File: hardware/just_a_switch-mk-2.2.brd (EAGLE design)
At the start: 22.9 x 17.8 mm, 13 parts, among them U1_ ROTARY_ENCODER_SWITCH, U2 Tiny85

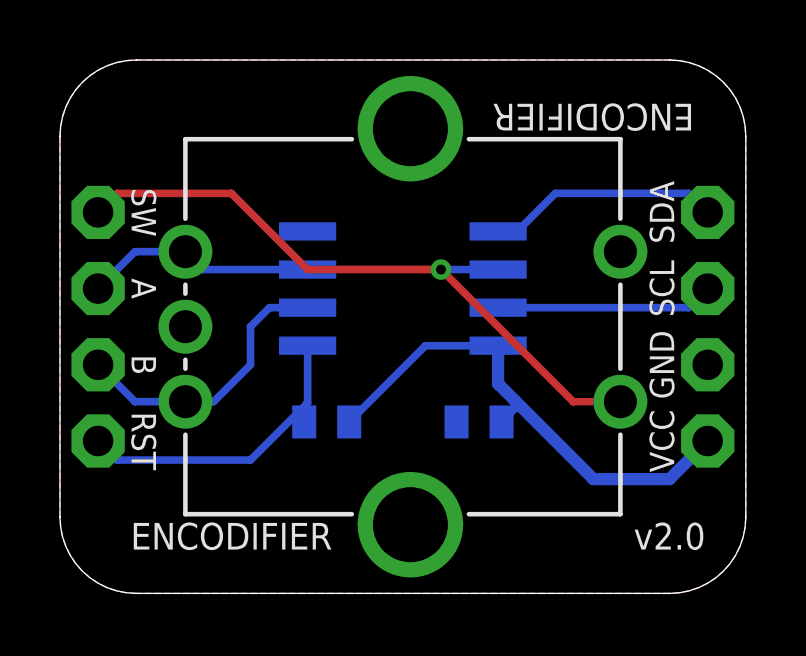
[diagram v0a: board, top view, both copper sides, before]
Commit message: have some boards, dawg
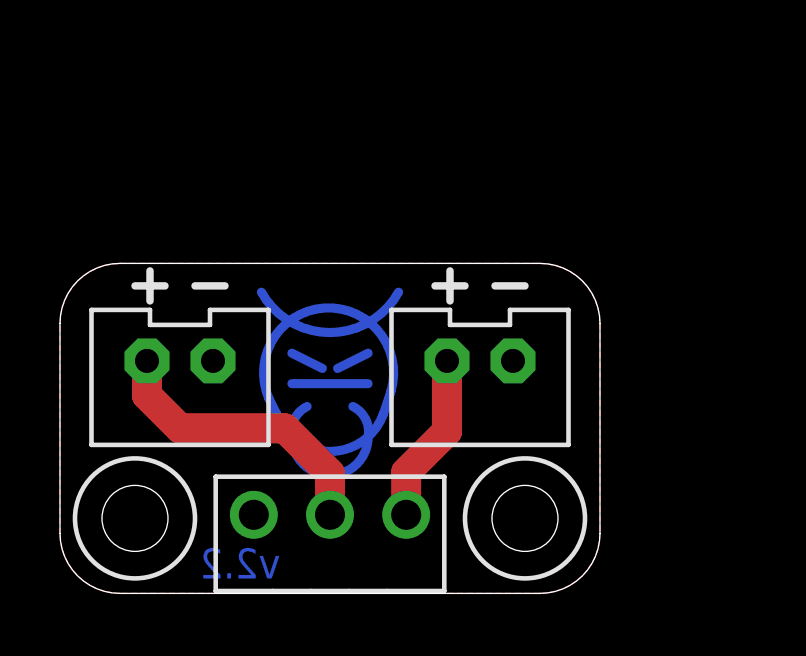
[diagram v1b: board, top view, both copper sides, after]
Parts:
- removed A, B, GND, RST, SCL, SDA, SW, VCC: M01PTH-1MM, a_parts:1X01-1MM-NS
- removed C1: 100n, a_parts:C0603-TIGHTER
- removed R1: 10k, a_parts:R0603-TIGHTER
- removed U1_: ROTARY_ENCODER_SWITCH, a_parts:ROTARY_ENCODER_SWITCH
- removed U2: Tiny85, a_parts:SO08-EIAJ
- added IN, OUT: M02JST-PH-VERT-R+, a_parts:JST-2-PH-VERT-PTH-R+
- added PWR: SWITCH-SPDTPTH-RA-2.54MM, a_parts:SPDT-RA-2.54MM
- added U$1: (no value), a_parts:COW_SMALL_METAL_NOTEXT
- FRAME1: device A_butts:DUMMY -> a_parts:DUMMY
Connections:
- removed net A: A.1, U1_.A, U2.3
- removed net B: B.1, U1_.B, U2.2
- removed net MOSI/SDA: SDA.1, U2.5
- removed net RST: R1.1, RST.1, U2.1
- removed net SCK/SCL: SCL.1, U2.7
- removed net SW: SW.1, U1_.SW1, U2.6
- new net N$1: IN.2, PWR.2
- net GND: now also IN.1, OUT.1; no longer C1.2, GND.1, U1_.C, U1_.SW2, U2.4
- net VCC: now also OUT.2, PWR.3; no longer C1.1, R1.2, U2.8, VCC.1
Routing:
- net SW: track 22.5 -> 0.00 mm, vias 1 -> 0
- net VCC: track 17.0 -> 5.69 mm
- net RST: track 10.5 -> 0.00 mm
- net N$1: track 0.00 -> 9.71 mm
- net B: track 9.54 -> 0.00 mm
- net MOSI/SDA: track 7.77 -> 0.00 mm
- net A: track 7.74 -> 0.00 mm
- net SCK/SCL: track 7.25 -> 0.00 mm
- removed copper zone on layer 16, net GND
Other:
- board size 22.9 x 17.8 mm -> 18 x 11 mm
- board text removed: "A"
- board text removed: "B"
- board text removed: "C"
- board text removed: "COM"
- board text removed: "ENCODIFIER"
- board text removed: "SW"
